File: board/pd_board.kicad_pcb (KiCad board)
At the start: 2 copper layers, 50 x 50 mm, 13 parts, among them P1 Vin Gnd, P2 OUT 1, P3 OUT 2, P4 OUT 3, P5 OUT 4, P6 OUT 5, P7 OUT 6, P8 OUT 7, P9 OUT 8

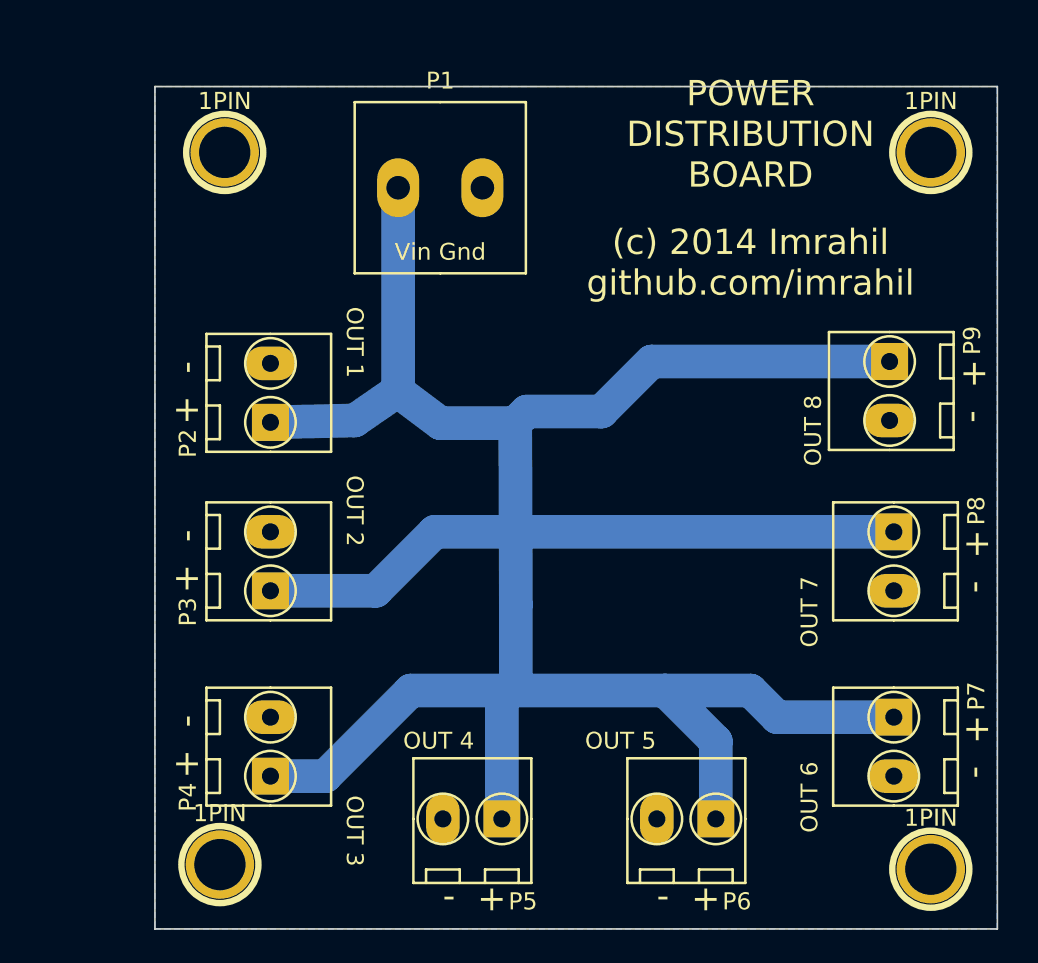
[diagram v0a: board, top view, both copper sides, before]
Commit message: Cleanup. Minor changes
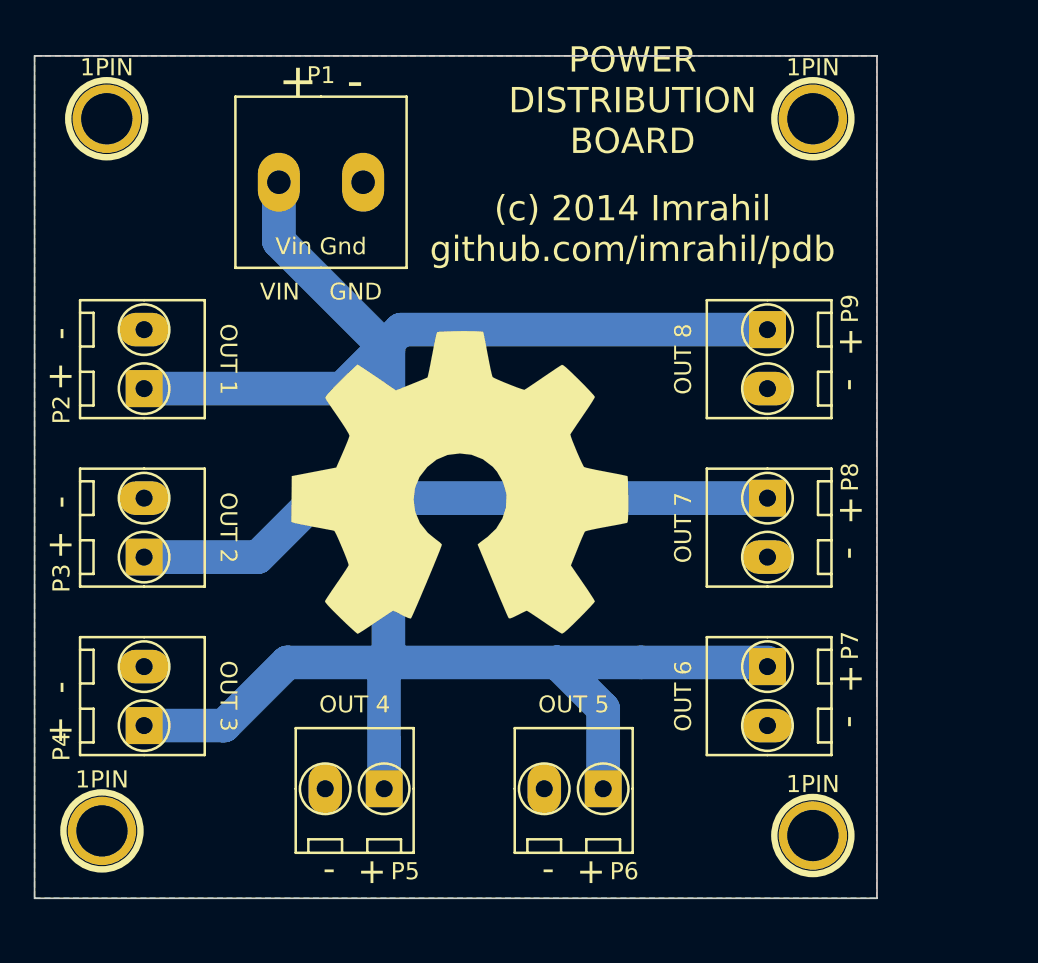
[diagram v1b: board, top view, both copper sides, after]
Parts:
- added G***: OSHW-logo_silkscreen-front_20mm, OSHW-logo_silkscreen-front_20mm, F.Cu at (135.2, 145.3)
- moved P4 8.08 mm to (116.5, 158.0)
- moved P7 8.08 mm to (153.5, 158.0)
- moved P2 7.76 mm to (116.5, 138.0)
- moved P3 7.76 mm to (116.5, 148.0)
- moved P8 7.76 mm to (153.5, 148.0)
- moved P9 7.49 mm to (153.5, 138.0)
- moved 1PIN 7.28 mm to (114.3, 123.7)
- moved 1PIN 7.28 mm to (156.2, 123.7)
- moved 1PIN 7.28 mm to (156.2, 166.3)
- moved 1PIN 7.28 mm to (114.0, 166.0)
- moved P5 7.21 mm to (129.0, 163.5)
- moved P1 7.09 mm to (127.0, 127.5)
- moved P6 6.92 mm to (142.0, 163.5)
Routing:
- added copper zone on F.Cu, net GND
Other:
- outline, holes or cut-outs redrawn
- board text added: "(c) 2014 Imrahil github.com/imrahil/pdb"
- board text added: "VIN GND"
- board text removed: "(c) 2014 Imrahil github.com/imrahil"
